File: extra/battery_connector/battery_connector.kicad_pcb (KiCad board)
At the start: 2 copper layers, 22 x 31 mm, 2 parts, among them J1 Conn_01x05_Socket, J3 Conn_01x10

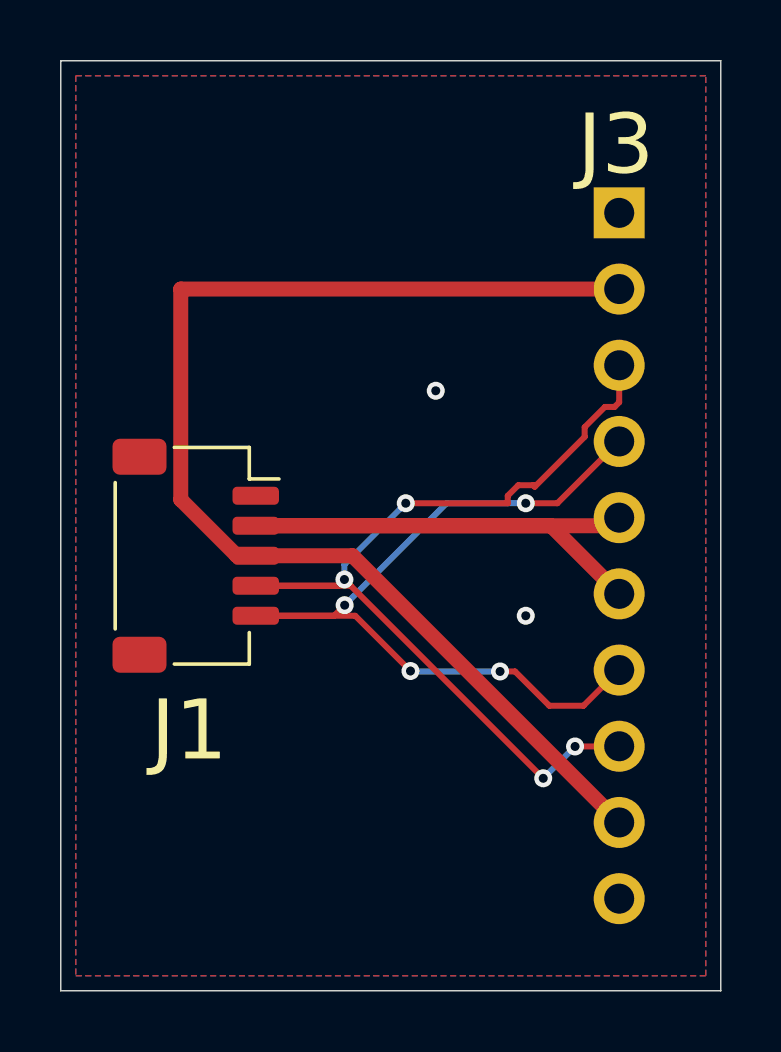
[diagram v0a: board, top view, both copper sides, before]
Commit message: Generated production files
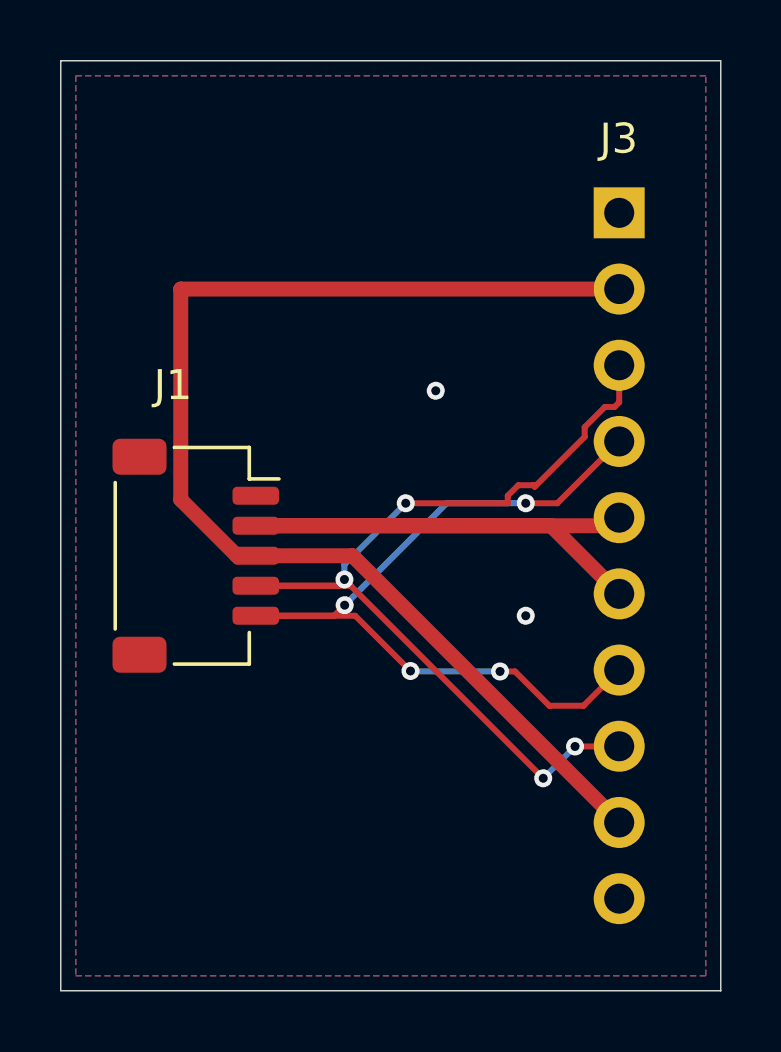
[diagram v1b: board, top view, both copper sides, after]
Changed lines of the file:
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@@
 		(tags "Through hole angled pin header THT 1x10 2.54mm single row")
 		(property "Reference" "J3"
-			(at -0.115 -2.27 0)
+			(at -0.015 -2.47 0)
 			(layer "F.SilkS")
 			(effects
 				(font
-					(size 2 2)
+					(size 1 1)
 					(thickness 0.15)
 				)
@@
 	)
 	(gr_text "J1"
-		(at 18 46 0)
+		(at 18.1 33.9 0)
 		(layer "F.SilkS")
 		(effects
 			(font
-				(size 2 2)
-				(thickness 0.1)
+				(size 1 1)
+				(thickness 0.15)
 			)
 			(justify left bottom)
